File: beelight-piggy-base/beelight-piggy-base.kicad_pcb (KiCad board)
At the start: 2 copper layers, 50 x 50 mm, 77 parts, among them J1 B_Le, J2 B_Ri, J3 USB_C_Receptacle_PowerOnly_6P, J4 WS2812_ext, J5 Conn_01x07_Pin, J7 DevSide, J8 B_Ri, J9 B_Le, Q1 AO3400A, U1 MCP73871, U2 BMA253, U3 TPS22917LDBV, U5 VEML3328, U6 TSOP382xx

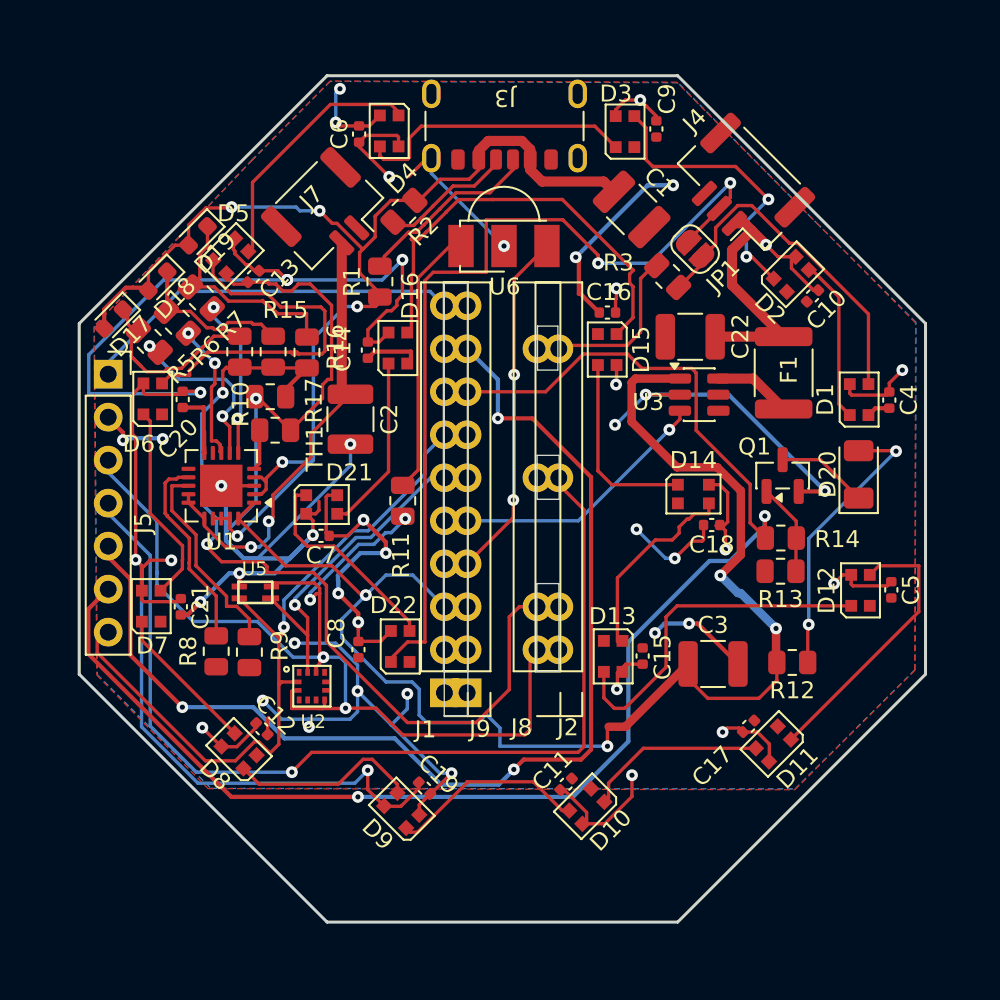
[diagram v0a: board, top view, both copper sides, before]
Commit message: pre jlc proto order
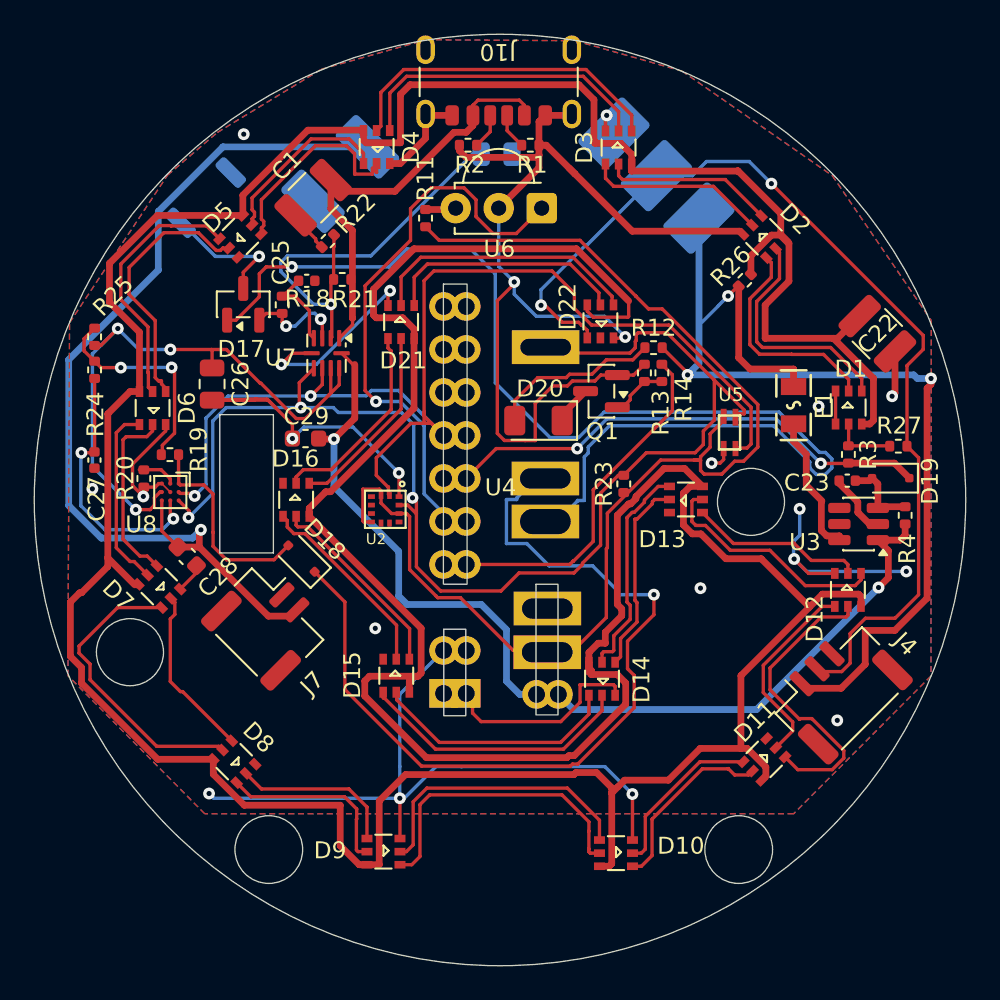
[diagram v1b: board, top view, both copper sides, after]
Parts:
- removed C10, C11, C12, C13, C14, C15, C16, C17, C18, C19, C20, C21, C4, C5, C6, C7, C8, C9: 100n, Capacitor_SMD:C_0402_1005Metric
- removed C2, C3: 4.7µF, Capacitor_SMD:C_1210_3225Metric
- removed J1, J9: B_Le, Connector_PinHeader_2.54mm:PinHeader_1x10_P2.54mm_Vertical
- removed J2, J8: B_Ri, Connector_PinHeader_2.54mm:PinHeader_1x10_P2.54mm_Vertical
- removed J5: Conn_01x07_Pin, Connector_PinSocket_2.54mm:PinSocket_1x07_P2.54mm_Vertical
- removed JP1: bypass_ws, Jumper:SolderJumper-2_P1.3mm_Open_RoundedPad1.0x1.5mm
- removed R10: 10k, Resistor_SMD:R_0805_2012Metric
- removed R15: 20k, Resistor_SMD:R_0805_2012Metric
- removed R16: 40k, Resistor_SMD:R_0805_2012Metric
- removed R17: 4k7, Resistor_SMD:R_0805_2012Metric
- removed R5, R6, R7, R8, R9: 470R, Resistor_SMD:R_0805_2012Metric
- removed U1: MCP73871, Package_DFN_QFN:QFN-20-1EP_4x4mm_P0.5mm_EP2.5x2.5mm
- added C23: 100nF, Capacitor_SMD:C_0402_1005Metric, F.Cu at (175.7, 94.2)
- added C25: 100nF, Capacitor_SMD:C_0402_1005Metric, F.Cu at (143.8, 82.4)
- added C26: 10uF, Capacitor_SMD:C_0805_2012Metric, F.Cu at (138.2, 88.5)
- added C27: 1uF, Capacitor_SMD:C_0402_1005Metric, F.Cu at (131.3, 93.0)
- added C28: 1uF, Capacitor_SMD:C_0603_1608Metric, F.Cu at (136.8, 98.7)
- added C29: 2.2uF, Capacitor_SMD:C_0603_1608Metric, F.Cu at (143.7, 91.7)
- added J10: USB C power only, Connector_USB:USB_C_Receptacle_GCT_USB4125-xx-x_6P_TopMnt_Horizontal, F.Cu at (155.2, 69.5)
- added J11: ExtWSSolderPads, Crystal:Resonator_SMD-3Pin_7.2x3.0mm_HandSoldering, B.Cu at (164.5, 76.2)
- added R18: 200k, Resistor_SMD:R_0402_1005Metric, F.Cu at (142.4, 83.8)
- added R19: 10k, Resistor_SMD:R_0402_1005Metric, F.Cu at (135.7, 92.7)
- added R20: 10k, Resistor_SMD:R_0402_1005Metric, F.Cu at (134.2, 94.1)
- added R21: 6.34k, Resistor_SMD:R_0402_1005Metric, F.Cu at (145.9, 82.3)
- added R22: 22.1k, Resistor_SMD:R_0402_1005Metric, F.Cu at (145.1, 80.0)
- added R23: 10k, Resistor_SMD:R_0402_1005Metric, F.Cu at (162.5, 94.4)
- added R24: 0R, Resistor_SMD:R_0402_1005Metric, F.Cu at (131.3, 87.7)
- added R25: 0R, Resistor_SMD:R_0402_1005Metric, F.Cu at (131.3, 85.7)
- added R26: 0R, Resistor_SMD:R_0402_1005Metric, F.Cu at (169.7, 82.4)
- added R27: 0R, Resistor_SMD:R_0402_1005Metric, F.Cu at (178.8, 92.2)
- added R4: 100k, Resistor_SMD:R_0402_1005Metric, F.Cu at (179.2, 96.3)
- added SW1: SW_Push, Button_Switch_SMD:SW_Push_SPST_NO_Alps_SKRK, B.Cu at (137.8, 77.5)
- added U4: rysta, beelight:rysta, F.Cu at (155.3, 95.4)
- added U7: MP2667, beelight:QFN-10_2x2mm_P0.5mm, F.Cu at (145.0, 86.7)
- added U8: BQ27421-G1, beelight:BGA-9_1.6x1.6mm_Layout3x3_P0.5mm, F.Cu at (135.8, 94.9)
- C1: value 10µF -> 10uF
- D1, D10, D11, D12, D13, D14, D15, D16, D2, D21, D22, D3, D4, D5, D6, D7, D8, D9: footprint LED_SMD:LED_WS2812B-2020_PLCC4_2.0x2.0mm -> EasyEDA_Lib:LED-SMD_6P-L2.2-W2.0_WS2816B-2020
- D17: value LED_Small -> BAT54C; footprint LED_SMD:LED_0603_1608Metric -> Package_TO_SOT_SMD:SOT-23
- D18, D19: value LED_Small -> BAT54J; footprint LED_SMD:LED_0603_1608Metric -> Diode_SMD:D_SOD-323F
- F1: footprint Fuse:Fuse_1812_4532Metric -> EasyEDA_Lib:F0805
- J3: value USB_C_Receptacle_PowerOnly_6P -> BatSolderPads; footprint Connector_USB:USB_C_Receptacle_GCT_USB4125-xx-x-0190_6P_TopMnt_Horizontal -> Diode_SMD:D_2114_3652Metric_Pad1.85x3.75mm_HandSolder; moved to B.Cu
- R1, R2: value 22k -> 5k1; footprint Resistor_SMD:R_0805_2012Metric -> Resistor_SMD:R_0402_1005Metric
- R11, R12, R13, R14, R3: footprint Resistor_SMD:R_0805_2012Metric -> Resistor_SMD:R_0402_1005Metric
- TH1: moved to B.Cu
- U2: footprint BMA253:LGA-12 -> beelight:LGA-12
- moved D19 43.3 mm to (178.3, 94.1), turned to 180 degrees
- moved J4 30.4 mm to (175.3, 106.6), turned to 45 degrees
- moved U5 29.8 mm to (168.4, 92.4), turned to 90 degrees
- moved J7 24.6 mm to (141.5, 102.7), turned to -45 degrees
- moved D15 22.9 mm to (149.1, 105.7), turned to 90 degrees
- moved D22 22.6 mm to (161.2, 84.8), turned to -90 degrees
- moved TH1 20.9 mm to (155.0, 74.9)
- moved R12 20.3 mm to (164.3, 86.3), turned to 0 degrees
- moved D20 19.2 mm to (157.5, 90.7), turned to 180 degrees
- moved C1 18.8 mm to (144.2, 77.5), turned to -135 degrees
- moved D18 18.5 mm to (143.5, 98.8), turned to 135 degrees
- moved R11 16.8 mm to (150.8, 78.7)
- moved R3 15.0 mm to (175.8, 92.7), turned to -90 degrees
- moved R13 14.2 mm to (163.8, 87.8), turned to 90 degrees
- moved D14 12.2 mm to (161.3, 105.9), turned to -90 degrees
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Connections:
- net Net-(J1-SCL) renamed SCL
- net Net-(J1-SDA) renamed SDA
- C22 pad 1: VLED -> Net-(D1-VDD)
- D1 pad 1: Net-(D1-DOUT) -> GND
- D1 pad 2: GND -> Net-(D1-DI)
- D1 pad 3: Net-(D1-DIN) -> Net-(D1-VDD)
- D1 pad 4: VLED -> Net-(D1-DO)
- D10 pad 1: Net-(D10-DOUT) -> Net-(D10-BI)
- D10 pad 2: GND -> Net-(D10-DI)
- D10 pad 3: Net-(D10-DIN) -> Net-(D1-VDD)
- D10 pad 4: VLED -> Net-(D10-DO)
- D11 pad 1: Net-(D11-DOUT) -> Net-(D10-BO)
- D11 pad 2: GND -> Net-(D10-DO)
- D11 pad 3: Net-(D10-DOUT) -> Net-(D1-VDD)
- D11 pad 4: VLED -> Net-(D11-DO)
- D12 pad 1: Net-(D12-DOUT) -> Net-(D11-BO)
- D12 pad 2: GND -> Net-(D11-DO)
- D12 pad 3: Net-(D11-DOUT) -> Net-(D1-VDD)
- D12 pad 4: VLED -> Net-(D12-DO)
- D13 pad 1: Net-(D13-DOUT) -> Net-(D12-BO)
- D13 pad 2: GND -> Net-(D12-DO)
- D13 pad 3: Net-(D12-DOUT) -> Net-(D1-VDD)
- D13 pad 4: VLED -> Net-(D13-DO)
- D14 pad 1: Net-(D14-DOUT) -> Net-(D13-BO)
- D14 pad 2: GND -> Net-(D13-DO)
- D14 pad 3: Net-(D13-DOUT) -> Net-(D1-VDD)
- D14 pad 4: VLED -> Net-(D14-DO)
- D15 pad 1: Net-(D15-DOUT) -> Net-(D14-BO)
- D15 pad 2: GND -> Net-(D14-DO)
- D15 pad 3: Net-(D14-DOUT) -> Net-(D1-VDD)
- D15 pad 4: VLED -> Net-(D15-DO)
- D16 pad 1: Net-(D16-DOUT) -> Net-(D15-BO)
- D16 pad 2: GND -> Net-(D15-DO)
- D16 pad 3: Net-(D15-DOUT) -> Net-(D1-VDD)
- D16 pad 4: VLED -> Net-(D16-DO)
- D17 pad 1: Net-(D17-K) -> WAKE
- D17 pad 2: VBUS -> Net-(U7-INT)
- D18 pad 1: Net-(D18-K) -> RST
- D18 pad 2: VBUS -> Net-(D18-A)
- D19 pad 1: Net-(D19-K) -> WS_DATA
- D19 pad 2: VBUS -> Net-(D19-A)
- D2 pad 1: Net-(D2-DOUT) -> Net-(D1-BO)
- D2 pad 2: GND -> Net-(D1-DO)
- D2 pad 3: Net-(D1-DOUT) -> Net-(D1-VDD)
- D2 pad 4: VLED -> Net-(D2-DO)
- D21 pad 1: Net-(D21-DOUT) -> Net-(D16-BO)
- D21 pad 2: GND -> Net-(D16-DO)
- D21 pad 3: Net-(D16-DOUT) -> Net-(D1-VDD)
- D21 pad 4: VLED -> Net-(D21-DO)
- D22 pad 1: Net-(D22-DOUT) -> Net-(D21-BO)
- D22 pad 2: GND -> Net-(D21-DO)
- D22 pad 3: Net-(D21-DOUT) -> Net-(D1-VDD)
- D22 pad 4: VLED -> Net-(D22-DO)
- D3 pad 1: Net-(D3-DOUT) -> Net-(D2-BO)
- D3 pad 2: GND -> Net-(D2-DO)
- D3 pad 3: Net-(D2-DOUT) -> Net-(D1-VDD)
- D3 pad 4: VLED -> Net-(D3-DO)
- D4 pad 1: Net-(D4-DOUT) -> Net-(D3-BO)
- D4 pad 2: GND -> Net-(D3-DO)
- D4 pad 3: Net-(D3-DOUT) -> Net-(D1-VDD)
- D4 pad 4: VLED -> Net-(D4-DO)
- D5 pad 1: Net-(D5-DOUT) -> Net-(D4-BO)
- D5 pad 2: GND -> Net-(D4-DO)
- D5 pad 3: Net-(D4-DOUT) -> Net-(D1-VDD)
- D5 pad 4: VLED -> Net-(D5-DO)
- D6 pad 1: Net-(D6-DOUT) -> Net-(D5-BO)
- D6 pad 2: GND -> Net-(D5-DO)
- D6 pad 3: Net-(D5-DOUT) -> Net-(D1-VDD)
- D6 pad 4: VLED -> Net-(D6-DO)
- D7 pad 1: Net-(D7-DOUT) -> Net-(D6-BO)
- D7 pad 2: GND -> Net-(D6-DO)
- D7 pad 3: Net-(D6-DOUT) -> Net-(D1-VDD)
- D7 pad 4: VLED -> Net-(D7-DO)
- D8 pad 1: Net-(D8-DOUT) -> Net-(D7-BO)
- D8 pad 2: GND -> Net-(D7-DO)
- D8 pad 3: Net-(D7-DOUT) -> Net-(D1-VDD)
- D8 pad 4: VLED -> Net-(D8-DO)
- D9 pad 1: Net-(D10-DIN) -> Net-(D8-BO)
- D9 pad 2: GND -> Net-(D8-DO)
- D9 pad 3: Net-(D8-DOUT) -> Net-(D1-VDD)
- D9 pad 4: VLED -> Net-(D10-DI)
- F1 pad 1: Net-(U3-VOUT) -> VLED
- F1 pad 2: VLED -> Net-(U3-VOUT)
- J4 pad 2: Net-(D22-DOUT) -> Net-(D22-DO)
- J7 pad 2: Net-(J7-Pin_2) -> BAT
- R1 pad 1: VBUS -> Net-(J10-CC1)
- R1 pad 2: Net-(J3-CC1) -> GND
- R12 pad 2: +5VP -> VLED
- R14 pad 1: Net-(J1-TXD) -> IR_TX
- R2 pad 1: VBUS -> GND
- R2 pad 2: Net-(J3-CC2) -> Net-(J10-CC2)
- R3 pad 1: Net-(J2-BUZ) -> Net-(D1-DI)
- R3 pad 2: Net-(D1-DIN) -> WS_DATA
- TH1 pad 1: Net-(U1-THERM) -> NTC
- U3 pad 3: Net-(J1-SCL2) -> Net-(D19-A)
- U6 pad 1: Net-(J1-SCLP) -> IR_RX
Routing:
- net Net-(D1-VDD): track 0.00 -> 289.4 mm
- net VLED: track 178.1 -> 62.0 mm, vias 23 -> 3
- net Net-(J1-TXD): track 86.1 -> 0.00 mm, vias 2 -> 0
- net WAKE: track 0.00 -> 70.7 mm, vias 0 -> 1
- net Net-(J1-RXD): track 66.4 -> 0.00 mm, vias 3 -> 0
- net Net-(D22-DO): track 0.00 -> 59.7 mm, vias 0 -> 2
- net Net-(J2-RST): track 58.4 -> 0.00 mm, vias 1 -> 0
- net BAT: track 0.00 -> 55.4 mm, vias 0 -> 1
- net SCL: track 19.6 -> 74.1 mm, vias 1 -> 3
- net Net-(D22-DOUT): track 53.1 -> 0.00 mm, vias 2 -> 0
- net RST: track 0.00 -> 50.6 mm, vias 0 -> 1
- net Net-(J2-ADC): track 50.1 -> 0.00 mm, vias 2 -> 0
- net VBUS: track 71.8 -> 24.6 mm, vias 5 -> 0
- net Net-(U8-SRX): track 0.00 -> 36.2 mm, vias 0 -> 3
- net IR_RX: track 0.00 -> 32.4 mm, vias 0 -> 1
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- added copper zone on B.Cu, net GND
- removed copper zone on B.Cu, net VLED
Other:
- board size 50 x 50 mm -> 55 x 55 mm
